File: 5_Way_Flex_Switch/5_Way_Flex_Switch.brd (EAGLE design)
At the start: 51 x 26.5 mm, 9 parts

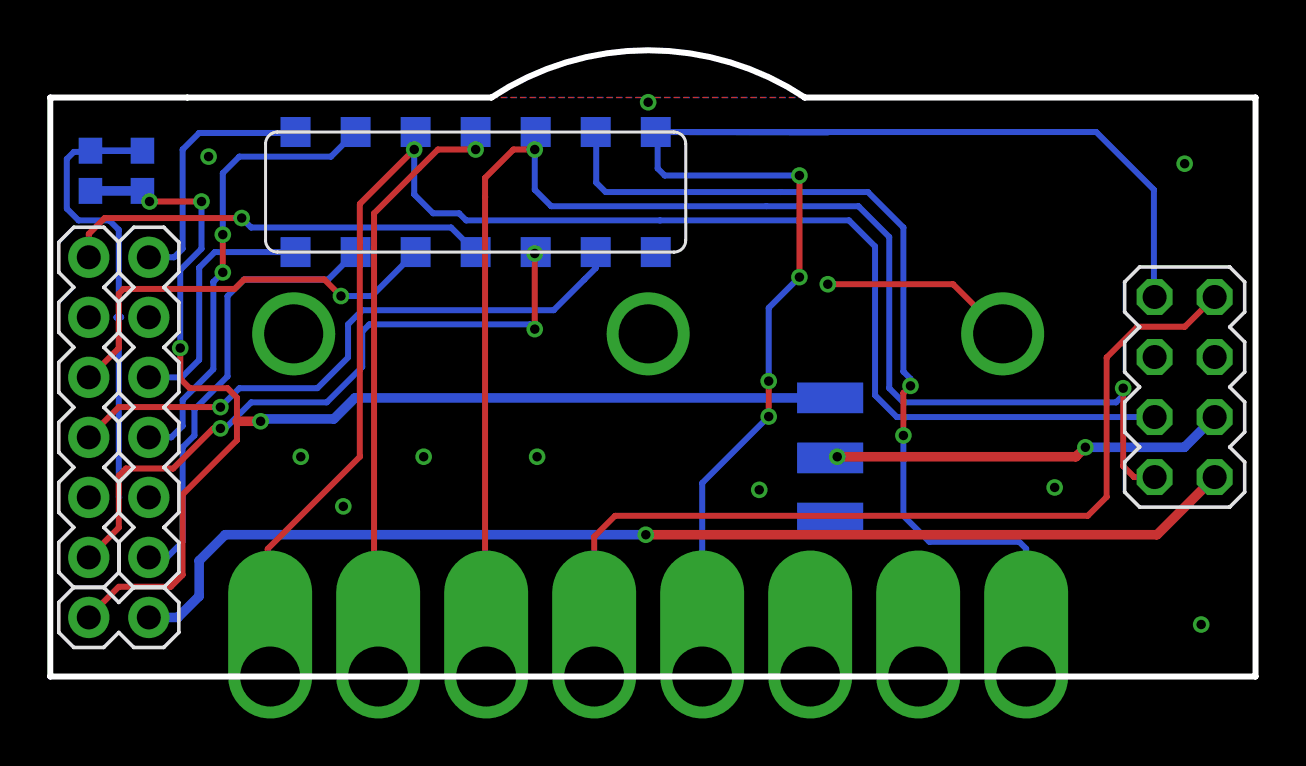
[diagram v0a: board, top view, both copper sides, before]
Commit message: Licenses
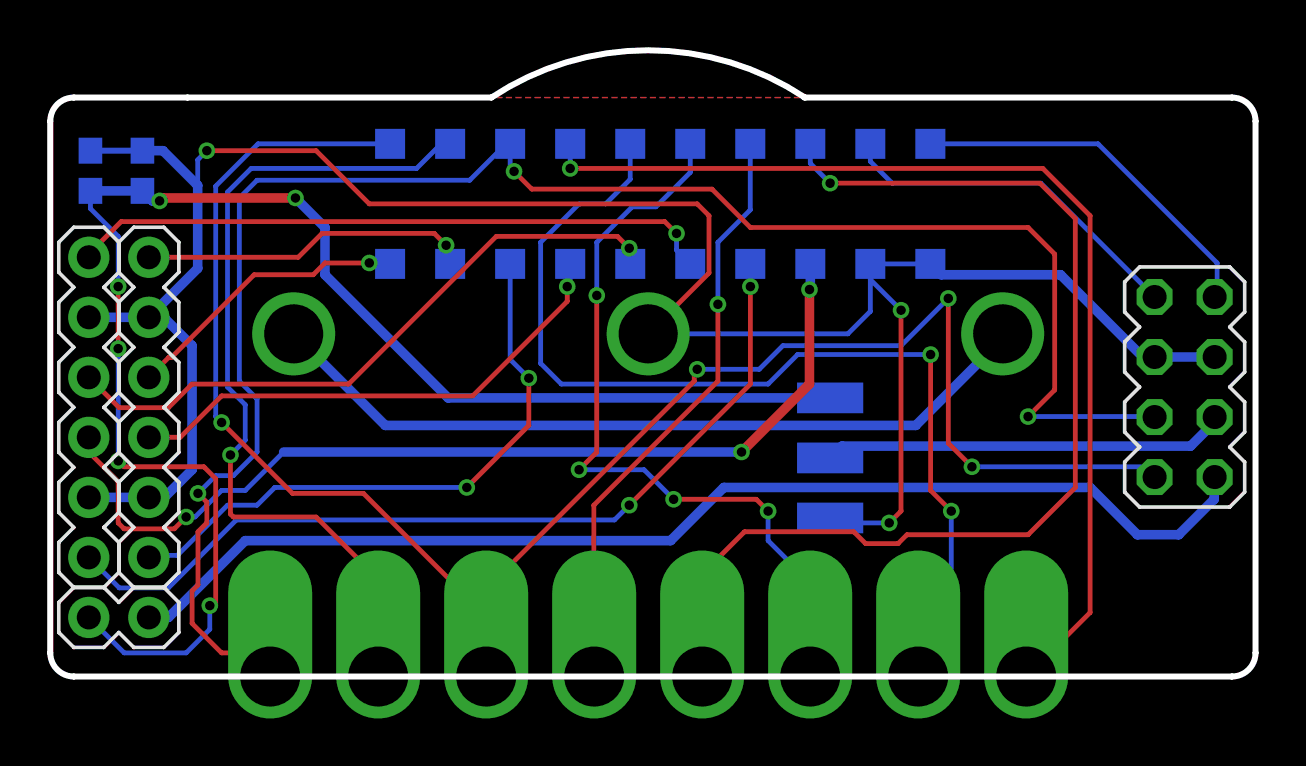
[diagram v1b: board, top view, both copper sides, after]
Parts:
- removed MOD1: CONFIGURATION_BRD, CYCFI_Module_castellated:CONFIGURATION_BRD
- added CB1: (no value), CYCFI_Module_castellated:CONFIGURATION_BRD_PADS
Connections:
- removed net M1: MOD1.M1, U$1.M1
- removed net N2: MOD1.N2, U$1.N2
- new net N$13: CB1.M1, U$1.M1
- new net N$15: CB1.N2, U$1.N2
- new net N$16: CB1.M2, U$1.M2
- new net N$17: CB1.B2, U$1.B2
- new net N$2: CB1.COM2, U$1.COM2
- new net N$3: CB1.COM1, U$1.COM1
- net 1-IC: now also CB1.1-IC; no longer MOD1.1-IC
- net 1-OC: now also CB1.1-OC; no longer MOD1.1-OC
- net 2-IC: now also CB1.2-IC; no longer MOD1.2-IC
- net 2-OC: now also CB1.2-OC; no longer MOD1.2-OC
- net 3-IC: now also CB1.3-IC; no longer MOD1.3-IC
- net 3-OC: now also CB1.3-OC; no longer MOD1.3-OC
- net 4-IC: now also CB1.4-IC; no longer MOD1.4-IC
- net 4-OC: now also CB1.4-OC; no longer MOD1.4-OC
- net B1: now also CB1.B1; no longer MOD1.B1
- net GND: now also CB1.GND, CB1.GND1; no longer MOD1.GND
- net IN+: now also CB1.OUT-; no longer U$1.COM1
- net IN-: now also CB1.OUT+; no longer MOD1.IN-, U$1.COM2
- net N1: now also CB1.N1; no longer MOD1.N1
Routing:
- net GND: track 30.1 -> 102.5 mm, vias 14 -> 4
- net IN-: track 64.5 -> 15.1 mm, vias 4 -> 0
- net N$2: track 0.00 -> 46.4 mm, vias 0 -> 1
- net N$15: track 0.00 -> 44.5 mm, vias 0 -> 1
- net N$16: track 0.00 -> 43.5 mm, vias 0 -> 2
- net N2: track 39.6 -> 0.00 mm, vias 2 -> 0
- net N$13: track 0.00 -> 36.0 mm, vias 0 -> 1
- net GND1: track 0.00 -> 33.3 mm, vias 0 -> 2
- net N$17: track 0.00 -> 32.9 mm, vias 0 -> 4
- net M1: track 25.8 -> 0.00 mm, vias 1 -> 0
- net N$3: track 0.00 -> 25.3 mm, vias 0 -> 1
- net IN+: track 39.8 -> 15.7 mm
- net 4-OC: track 26.2 -> 41.1 mm, vias 1 -> 3
- net N1: track 63.8 -> 76.7 mm, vias 2 -> 4
- net VBATT: track 54.3 -> 65.3 mm, vias 4 -> 6
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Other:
- outline, holes or cut-outs redrawn
